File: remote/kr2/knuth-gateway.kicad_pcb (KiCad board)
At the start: 2 copper layers, 69.1 x 80.6 mm, 21 parts, among them J1 FeatherLora1, J10 Screw_Terminal_01x02, J11 Screw_Terminal_01x02, J2 FeatherLora2, J3 Conn_01x02_Female, J4 Conn_01x02_Female, J5 Screw_Terminal_01x03, J6 Screw_Terminal_01x03, J7 Conn_01x03_Female, J8 Conn_01x02_Female, J9 Conn_01x02_Female, U4 tpl5111

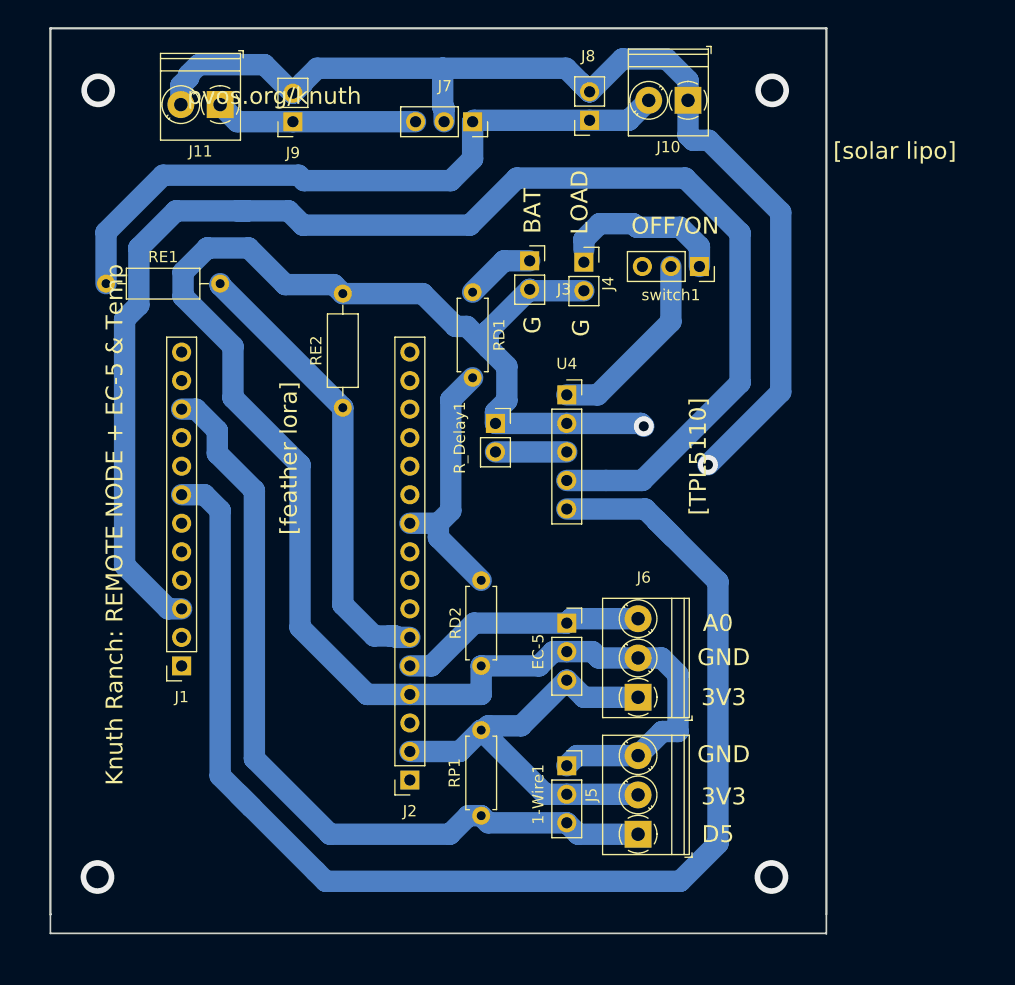
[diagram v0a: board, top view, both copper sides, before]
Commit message: update
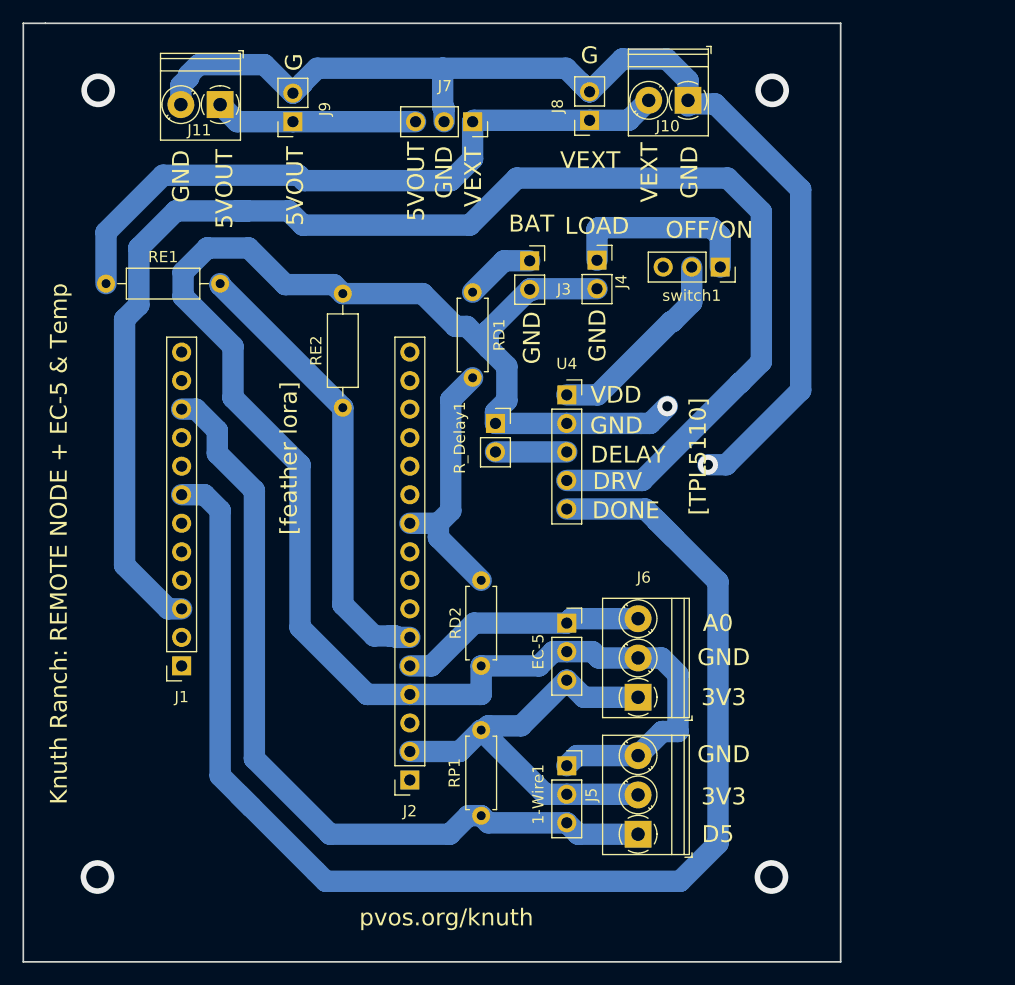
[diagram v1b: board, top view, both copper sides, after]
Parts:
- moved switch1 1.85 mm to (266.4, 67.4)
- moved J4 1.18 mm to (255.4, 66.8)
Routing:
- net GND: track 257.2 -> 263.9 mm
- net VBUS: track 127.9 -> 131.7 mm
- net LOAD: track 14.4 -> 16.9 mm
- net SWITCHED_LOAD: track 16.9 -> 17.7 mm
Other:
- board size 69.1 x 80.6 mm -> 72.8 x 83.6 mm
- board text added: "5VOUT"
- board text added: "DELAY"
- board text added: "DONE"
- board text added: "DRV"
- board text added: "VDD"
- board text added: "VEXT"
- board text removed: "[solar lipo]"
